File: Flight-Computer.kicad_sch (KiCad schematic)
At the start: 6 parts, among them U1 STM32U575RIT6, U2 STM32L552CCU6, U3 BNO055, U4 MS5611-01BA, U5 STM32L552CCUx

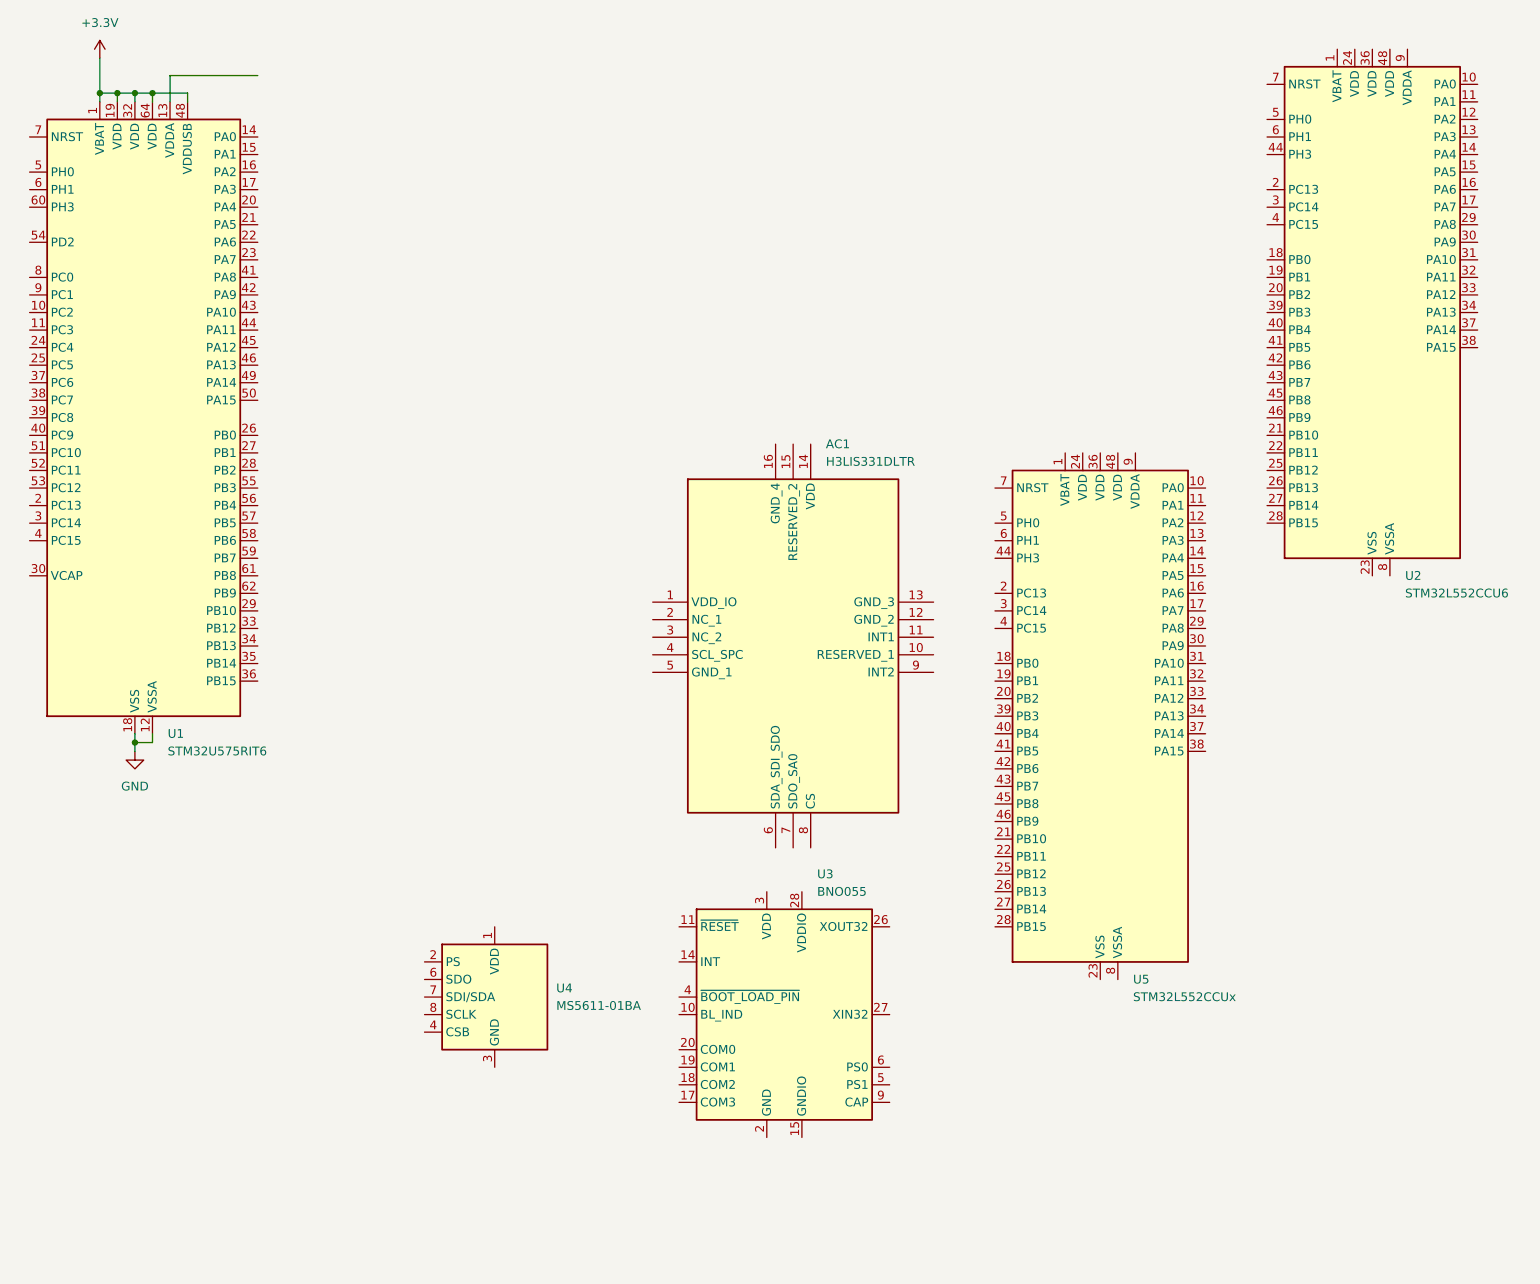
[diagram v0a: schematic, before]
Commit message: Added RF chips and Pages in Sch.
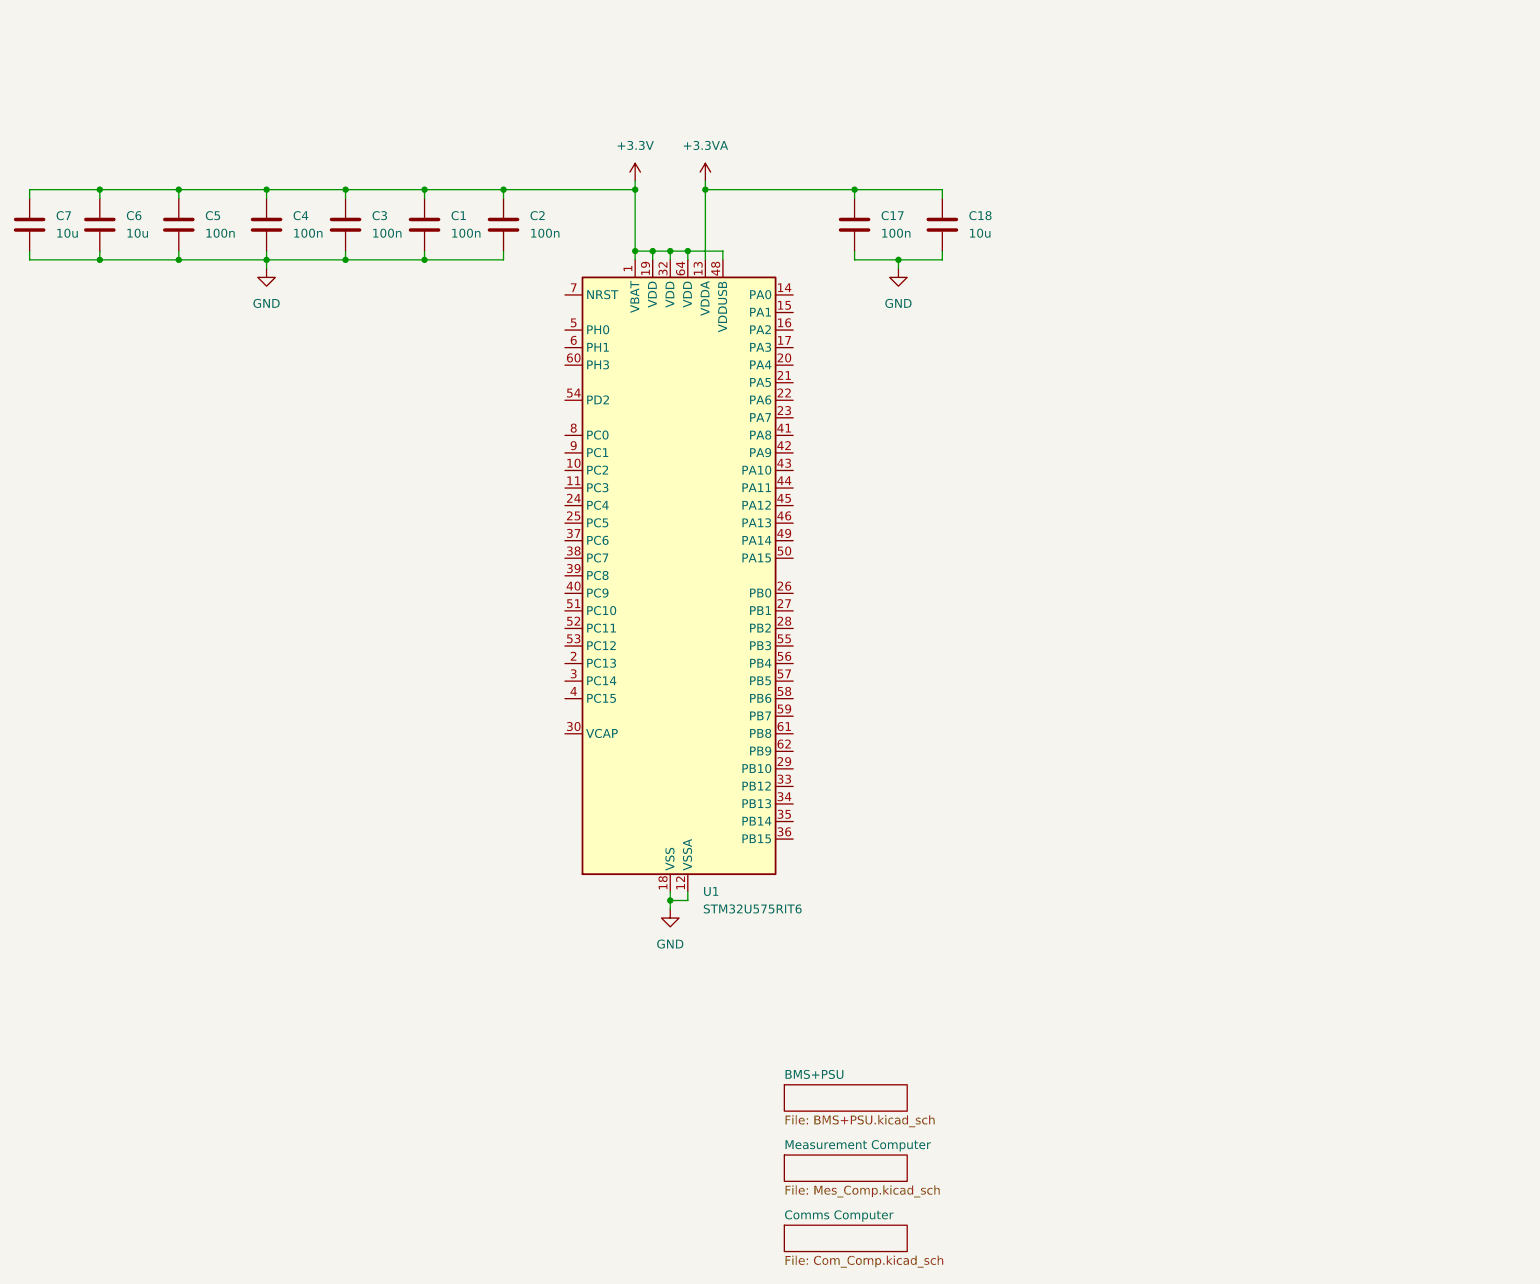
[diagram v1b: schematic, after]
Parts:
- removed AC1: H3LIS331DLTR, LIS3DHTR, symbol H3LIS331DLTR:H3LIS331DLTR
- removed U2: STM32L552CCU6, Package_DFN_QFN:QFN-48-1EP_7x7mm_P0.5mm_EP5.6x5.6mm, symbol MCU_ST_STM32L5:STM32L552CCUx
- removed U3: BNO055, Package_LGA:LGA-28_5.2x3.8mm_P0.5mm, symbol Sensor_Motion:BNO055
- removed U4: MS5611-01BA, Package_LGA:LGA-8_3x5mm_P1.25mm, symbol Sensor_Pressure:MS5611-01BA
- removed U5: STM32L552CCUx, Package_DFN_QFN:QFN-48-1EP_7x7mm_P0.5mm_EP5.6x5.6mm, symbol MCU_ST_STM32L5:STM32L552CCUx
- added C1, C17, C2, C3, C4, C5: 100n, symbol Device:C
- added C18, C6, C7: 10u, symbol Device:C
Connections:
- net +3.3V: now also C1.1, C2.1, C3.1, C4.1, C5.1, C6.1, C7.1
- net GND: now also C1.2, C17.2, C18.2, C2.2, C3.2, C4.2, C5.2, C6.2, C7.2
- net +3.3VA: now reaches U1.13 (VDDA)
- net +3.3VA: now also C17.1, C18.1
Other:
- added sheet BMS+PSU (BMS+PSU.kicad_sch)
- added sheet Comms Computer (Com_Comp.kicad_sch)
- added sheet Measurement Computer (Mes_Comp.kicad_sch)
- moved on the sheet: U1
